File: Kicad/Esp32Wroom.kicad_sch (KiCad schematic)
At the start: 34 parts, among them J1 Conn_01x08_Socket, J2 Conn_01x08_Pin, J3 Conn_01x10_Socket, J4 Conn_01x10_Pin, J5 Conn_01x05_Socket, J6 Conn_01x02_Socket, J7 Conn_01x05_Pin, J8 Conn_01x02_Pin, M1 Fan, Q1 TIP120, Q2 TIP120, Q3 TIP120, Q4 TIP120, Q5 TIP120, Q6 TIP120, SW1 <, SW2 Ok, SW3 >, U1 ESP32-WROOM, U2 ST7789, U3 DHT11

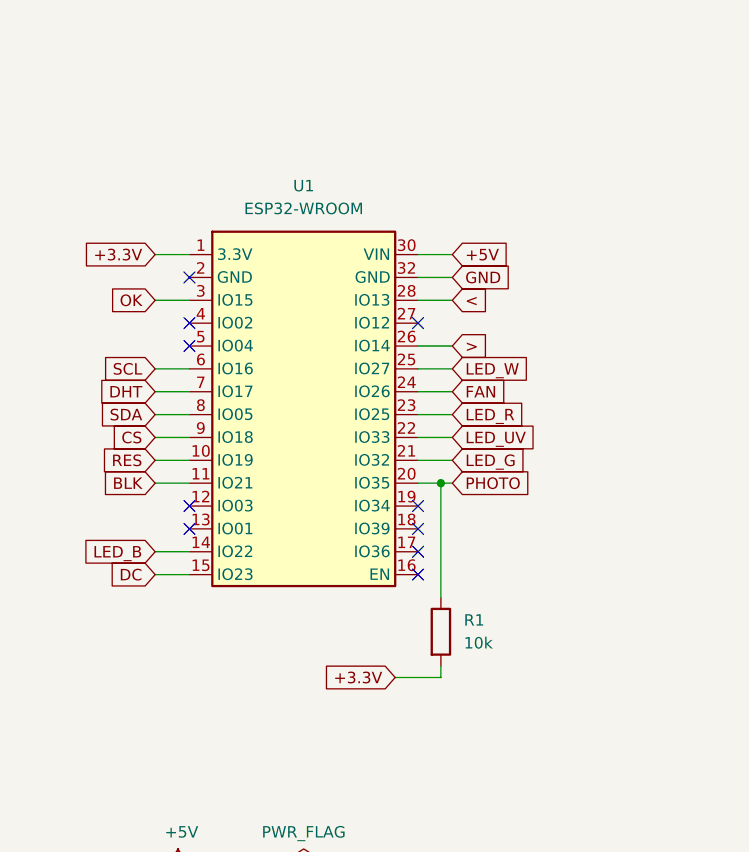
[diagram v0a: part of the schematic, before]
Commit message: uff02
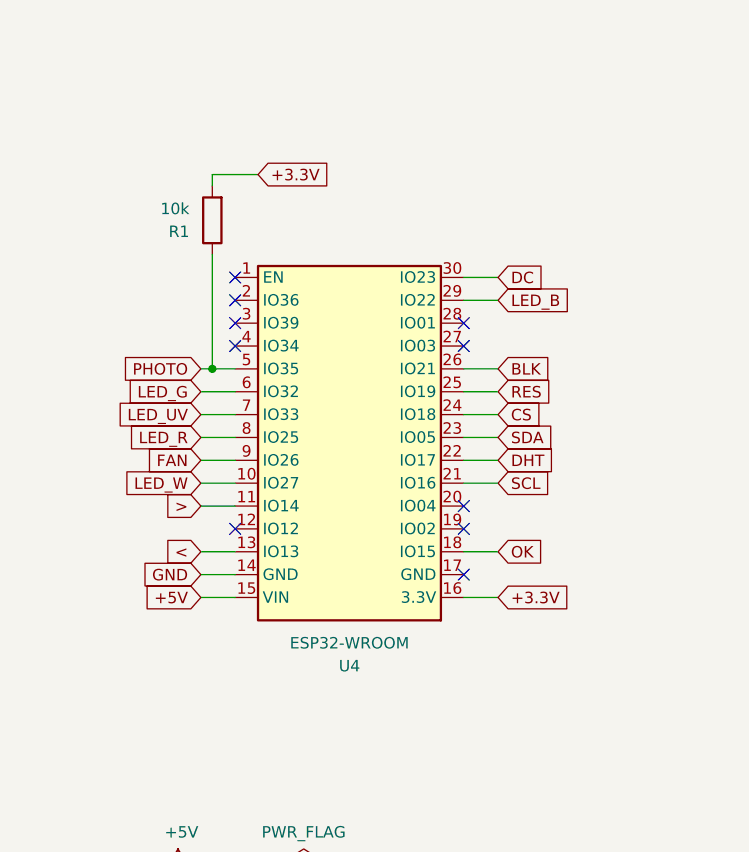
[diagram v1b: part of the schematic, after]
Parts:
- removed U1: ESP32-WROOM, ESP32 30 pin, symbol Esp32-rescue:ESP32-WROOM
- added U4: ESP32-WROOM, ESP32 30 pin, symbol Esp32-rescue:ESP32-WROOM
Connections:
- net +3.3V: now also U4.16 (3.3V)
- net +5V: now also U4.15 (VIN)
- net <: now also U4.13 (IO13)
- net >: now also U4.11 (IO14)
- net BLK: now also U4.26 (IO21)
- net CS: now also U4.24 (IO18)
- net DC: now also U4.30 (IO23)
- net DHT: now also U4.22 (IO17)
- net FAN: now also U4.9 (IO26)
- net GND: now also U4.14 (GND)
- net LED_B: now also U4.29 (IO22)
- net LED_G: now also U4.6 (IO32)
- net LED_R: now also U4.8 (IO25)
- net LED_UV: now also U4.7 (IO33)
- net LED_W: now also U4.10 (IO27)
- net OK: now also U4.18 (IO15)
- net PHOTO: now also U4.5 (IO35)
- net RES: now also U4.25 (IO19)
- net SCL: now also U4.21 (IO16)
- net SDA: now also U4.23 (IO05)
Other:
- moved on the sheet: R1

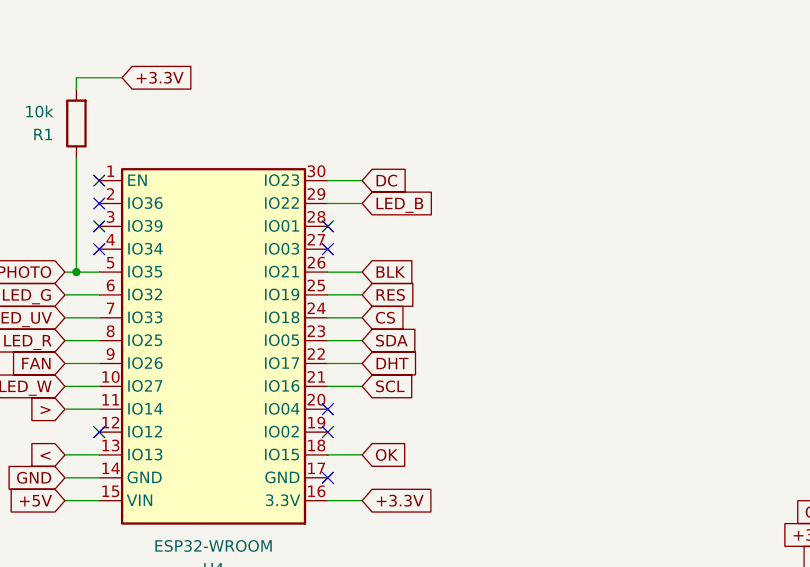
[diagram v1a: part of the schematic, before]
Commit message: casa03
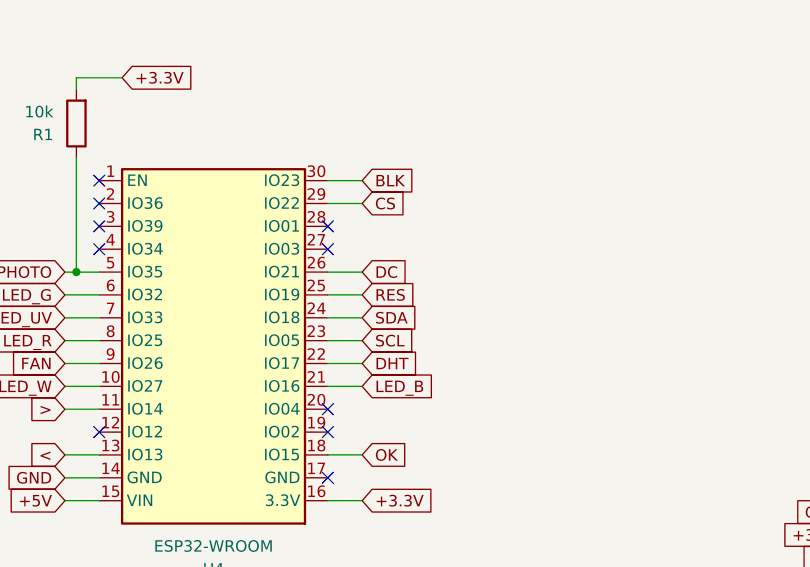
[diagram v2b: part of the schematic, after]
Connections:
- net BLK: now also U4.30 (IO23); no longer U4.26 (IO21)
- net CS: now also U4.29 (IO22); no longer U4.24 (IO18)
- net DC: now also U4.26 (IO21); no longer U4.30 (IO23)
- net LED_B: now also U4.21 (IO16); no longer U4.29 (IO22)
- net SCL: now also U4.23 (IO05); no longer U4.21 (IO16)
- net SDA: now also U4.24 (IO18); no longer U4.23 (IO05)
